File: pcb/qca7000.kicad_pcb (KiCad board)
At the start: 2 copper layers, 76 x 68.4 mm, 113 parts, among them J1 Conn_01x04_Pin, J2 Conn_01x08_Pin, J3 12V_in, U1 25Q16, U2 XL1509-5.0, U3 AMS1117-3.3, U4 AMS1117-3.3, Y1 25MHz

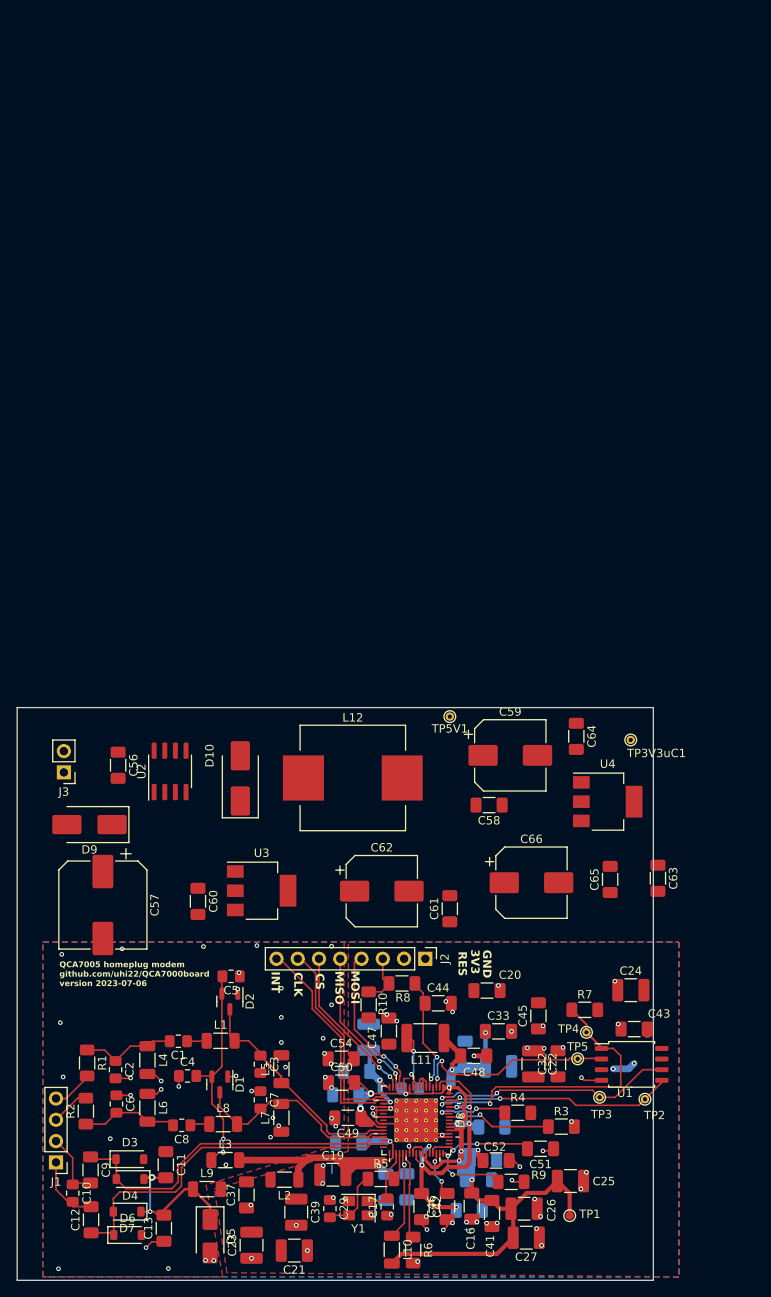
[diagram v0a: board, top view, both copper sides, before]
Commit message: added sheets for inputs and outputs. layout draft.
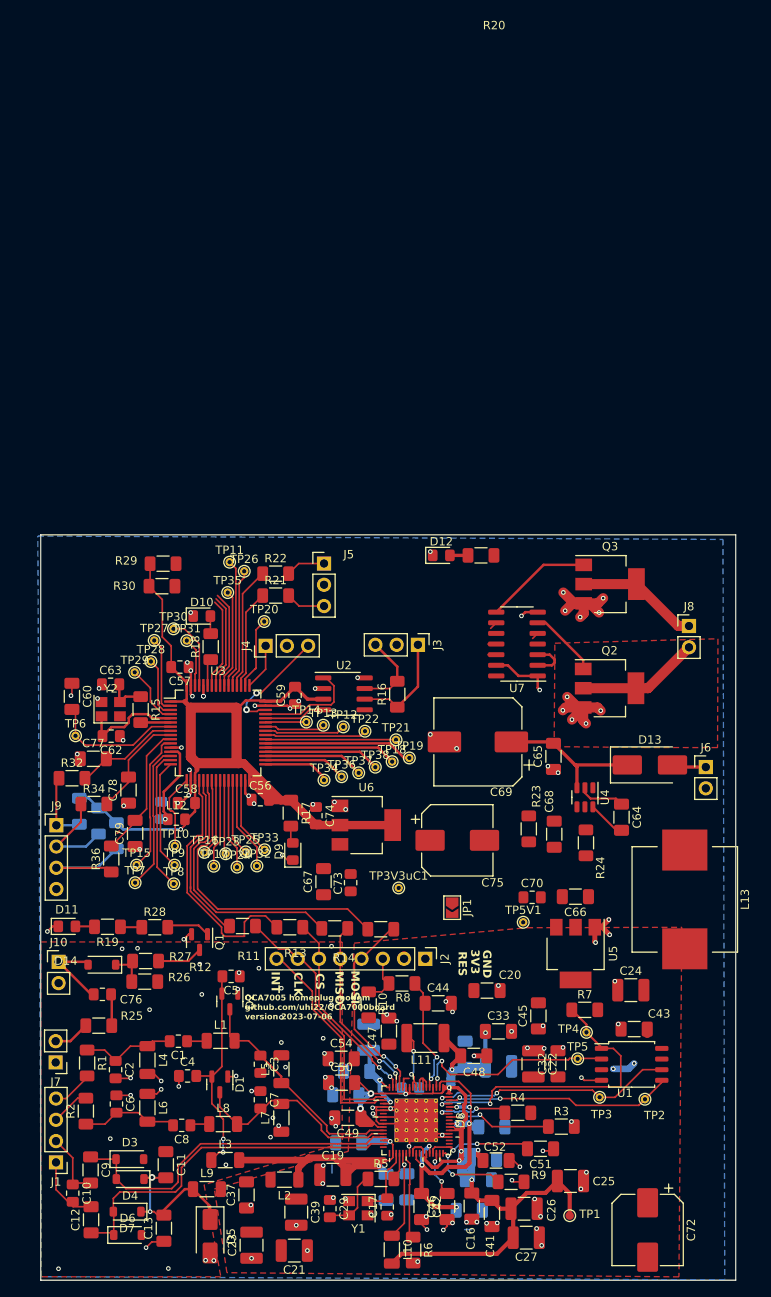
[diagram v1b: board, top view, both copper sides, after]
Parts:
- added C67: 22uF, Capacitor_SMD:C_1206_3216Metric_Pad1.33x1.80mm_HandSolder, F.Cu at (154.9, 81.5)
- added C68: 68pF, Capacitor_SMD:C_1206_3216Metric_Pad1.33x1.80mm_HandSolder, F.Cu at (182.5, 75.8)
- added C69: 470uF, Capacitor_SMD:CP_Elec_10x10, F.Cu at (173.4, 64.8)
- added C70: 100nF, Capacitor_SMD:C_0805_2012Metric_Pad1.18x1.45mm_HandSolder, F.Cu at (179.8, 83.3)
- added C72: 100uF, Capacitor_SMD:CP_Elec_8x10, F.Cu at (193.6, 123.1)
- added C73: 100nF, Capacitor_SMD:C_0805_2012Metric_Pad1.18x1.45mm_HandSolder, F.Cu at (158.2, 81.6)
- added C74: 100nF, Capacitor_SMD:C_0805_2012Metric_Pad1.18x1.45mm_HandSolder, F.Cu at (154.0, 73.6)
- added C75: 100uF, Capacitor_SMD:CP_Elec_8x10, F.Cu at (170.9, 76.5)
- added C76: 1nF, Capacitor_SMD:C_0805_2012Metric_Pad1.18x1.45mm_HandSolder, F.Cu at (128.5, 94.9)
- added C77: 100nF, Capacitor_SMD:C_1206_3216Metric_Pad1.33x1.80mm_HandSolder, F.Cu at (127.4, 66.8)
- added C78: 100nF, Capacitor_SMD:C_1206_3216Metric_Pad1.33x1.80mm_HandSolder, F.Cu at (131.6, 70.5)
- added C79: 100nF, Capacitor_SMD:C_1206_3216Metric_Pad1.33x1.80mm_HandSolder, F.Cu at (132.4, 75.7)
- added D11: LED, LED_SMD:LED_0805_2012Metric_Pad1.15x1.40mm_HandSolder, F.Cu at (124.3, 86.8)
- added D12: LED, LED_SMD:LED_0805_2012Metric_Pad1.15x1.40mm_HandSolder, F.Cu at (169.0, 42.5)
- added D13: SS54B-HF, Diode_SMD:D_SMB_Handsoldering, F.Cu at (193.9, 67.5)
- added D14: 1N4148W, Diode_SMD:D_SOD-123, F.Cu at (128.4, 91.4)
- added J10: CP/PE, Connector_PinHeader_2.54mm:PinHeader_1x02_P2.54mm_Vertical, F.Cu at (123.3, 91.0)
- added J4: DEBUG, Connector_PinHeader_2.54mm:PinHeader_1x03_P2.54mm_Vertical, F.Cu at (148.0, 53.3)
- added J5: UART, Connector_PinHeader_2.54mm:PinHeader_1x03_P2.54mm_Vertical, F.Cu at (155.0, 43.5)
- added J6: 12V_in, Connector_PinHeader_2.54mm:PinHeader_1x02_P2.54mm_Vertical, F.Cu at (200.6, 67.8)
- added J7: RF, Connector_PinHeader_2.54mm:PinHeader_1x02_P2.54mm_Vertical, F.Cu at (122.9, 103.1)
- added J8: CONTACTORS, Connector_PinHeader_2.54mm:PinHeader_1x02_P2.54mm_Vertical, F.Cu at (198.6, 50.9)
- added J9: Temps, Connector_PinHeader_2.54mm:PinHeader_1x04_P2.54mm_Vertical, F.Cu at (123.0, 74.7)
- added JP1: SolderJumper3V3together, Jumper:SolderJumper-2_P1.3mm_Open_TrianglePad1.0x1.5mm, F.Cu at (170.3, 84.6)
- added L13: 10uH, Inductor_SMD:L_Wuerth_WE-PD-Typ-LS_Handsoldering, F.Cu at (198.1, 83.6)
- added Q1: BC846, Package_TO_SOT_SMD:SOT-23, F.Cu at (140.1, 88.7)
- added Q2: NCV8402xST, Package_TO_SOT_SMD:SOT-223, F.Cu at (189.1, 58.4)
- added Q3: NCV8402xST, Package_TO_SOT_SMD:SOT-223, F.Cu at (189.2, 45.9)
- added R11: 220, Resistor_SMD:R_1206_3216Metric_Pad1.30x1.75mm_HandSolder, F.Cu at (150.9, 86.9)
- added R12: 220, Resistor_SMD:R_1206_3216Metric_Pad1.30x1.75mm_HandSolder, F.Cu at (145.2, 86.8)
- added R13: 220, Resistor_SMD:R_1206_3216Metric_Pad1.30x1.75mm_HandSolder, F.Cu at (156.3, 87.0)
- added R14: 220, Resistor_SMD:R_1206_3216Metric_Pad1.30x1.75mm_HandSolder, F.Cu at (161.8, 87.2)
- added R15: 33, Resistor_SMD:R_1206_3216Metric_Pad1.30x1.75mm_HandSolder, F.Cu at (133.1, 60.9)
- added R16: 1k, Resistor_SMD:R_1206_3216Metric_Pad1.30x1.75mm_HandSolder, F.Cu at (163.7, 59.1)
- added R17: 1k, Resistor_SMD:R_1206_3216Metric_Pad1.30x1.75mm_HandSolder, F.Cu at (151.0, 73.3)
- added R18: 1k, Resistor_SMD:R_1206_3216Metric_Pad1.30x1.75mm_HandSolder, F.Cu at (141.4, 53.4)
- added R19: 1k, Resistor_SMD:R_1206_3216Metric_Pad1.30x1.75mm_HandSolder, F.Cu at (129.1, 86.9)
- added R20: 1k, Resistor_SMD:R_1206_3216Metric_Pad1.30x1.75mm_HandSolder, F.Cu at (173.7, 42.5)
- added R21: 220, Resistor_SMD:R_1206_3216Metric_Pad1.30x1.75mm_HandSolder, F.Cu at (149.2, 47.3)
- added R22: 220, Resistor_SMD:R_1206_3216Metric_Pad1.30x1.75mm_HandSolder, F.Cu at (149.2, 44.7)
- added R23: 10k, Resistor_SMD:R_1206_3216Metric_Pad1.30x1.75mm_HandSolder, F.Cu at (179.4, 75.2)
- added R24: 10k, Resistor_SMD:R_1206_3216Metric_Pad1.30x1.75mm_HandSolder, F.Cu at (186.3, 76.8)
- added R25: 180, Resistor_SMD:R_1206_3216Metric_Pad1.30x1.75mm_HandSolder, F.Cu at (128.1, 98.7)
- added R26: 2k7, Resistor_SMD:R_1206_3216Metric_Pad1.30x1.75mm_HandSolder, F.Cu at (133.6, 93.4)
- added R27: 1k2, Resistor_SMD:R_1206_3216Metric_Pad1.30x1.75mm_HandSolder, F.Cu at (133.7, 91.0)
- added R28: 10k, Resistor_SMD:R_1206_3216Metric_Pad1.30x1.75mm_HandSolder, F.Cu at (134.8, 86.9)
- added R29: 10k, Resistor_SMD:R_1206_3216Metric_Pad1.30x1.75mm_HandSolder, F.Cu at (135.8, 43.5)
- added R30: 10k, Resistor_SMD:R_1206_3216Metric_Pad1.30x1.75mm_HandSolder, F.Cu at (135.6, 46.2)
- added R31: 10k, Resistor_SMD:R_1206_3216Metric_Pad1.30x1.75mm_HandSolder, B.Cu at (125.8, 73.0)
- added R32: 47k, Resistor_SMD:R_1206_3216Metric_Pad1.30x1.75mm_HandSolder, F.Cu at (124.9, 69.1)
- added R33: 10k, Resistor_SMD:R_1206_3216Metric_Pad1.30x1.75mm_HandSolder, B.Cu at (128.0, 74.2)
- added R34: 47k, Resistor_SMD:R_1206_3216Metric_Pad1.30x1.75mm_HandSolder, F.Cu at (127.5, 72.2)
- added R35: 10k, Resistor_SMD:R_1206_3216Metric_Pad1.30x1.75mm_HandSolder, B.Cu at (130.2, 76.0)
- added R36: 47k, Resistor_SMD:R_1206_3216Metric_Pad1.30x1.75mm_HandSolder, F.Cu at (129.6, 78.8)
- added TP10: ~, TestPoint:TestPoint_THTPad_D1.0mm_Drill0.5mm, F.Cu at (137.2, 77.2)
- added TP11: ~, TestPoint:TestPoint_THTPad_D1.0mm_Drill0.5mm, F.Cu at (143.7, 43.3)
- added TP12: ~, TestPoint:TestPoint_THTPad_D1.0mm_Drill0.5mm, F.Cu at (157.3, 63.0)
- added TP13: ~, TestPoint:TestPoint_THTPad_D1.0mm_Drill0.5mm, F.Cu at (154.9, 62.8)
- added TP14: ~, TestPoint:TestPoint_THTPad_D1.0mm_Drill0.5mm, F.Cu at (152.9, 62.4)
- added TP15: ~, TestPoint:TestPoint_THTPad_D1.0mm_Drill0.5mm, F.Cu at (132.6, 79.5)
- added TP16: ~, TestPoint:TestPoint_THTPad_D1.0mm_Drill0.5mm, F.Cu at (140.7, 78.0)
- added TP17: ~, TestPoint:TestPoint_THTPad_D1.0mm_Drill0.5mm, F.Cu at (141.8, 79.6)
- added TP18: ~, TestPoint:TestPoint_THTPad_D1.0mm_Drill0.5mm, F.Cu at (163.1, 67.1)
- added TP19: ~, TestPoint:TestPoint_THTPad_D1.0mm_Drill0.5mm, F.Cu at (165.2, 66.7)
- added TP20: ~, TestPoint:TestPoint_THTPad_D1.0mm_Drill0.5mm, F.Cu at (147.8, 50.4)
- added TP21: ~, TestPoint:TestPoint_THTPad_D1.0mm_Drill0.5mm, F.Cu at (163.6, 64.5)
- added TP22: ~, TestPoint:TestPoint_THTPad_D1.0mm_Drill0.5mm, F.Cu at (159.9, 63.5)
- added TP23: ~, TestPoint:TestPoint_THTPad_D1.0mm_Drill0.5mm, F.Cu at (143.2, 78.1)
- added TP24: ~, TestPoint:TestPoint_THTPad_D1.0mm_Drill0.5mm, F.Cu at (144.6, 79.7)
- added TP25: ~, TestPoint:TestPoint_THTPad_D1.0mm_Drill0.5mm, F.Cu at (145.6, 77.9)
- added TP26: ~, TestPoint:TestPoint_THTPad_D1.0mm_Drill0.5mm, F.Cu at (145.4, 44.4)
- added TP27: ~, TestPoint:TestPoint_THTPad_D1.0mm_Drill0.5mm, F.Cu at (134.7, 52.6)
- added TP28: ~, TestPoint:TestPoint_THTPad_D1.0mm_Drill0.5mm, F.Cu at (134.3, 55.2)
- added TP29: ~, TestPoint:TestPoint_THTPad_D1.0mm_Drill0.5mm, F.Cu at (132.4, 56.5)
- added TP30: ~, TestPoint:TestPoint_THTPad_D1.0mm_Drill0.5mm, F.Cu at (137.0, 51.3)
- added TP31: ~, TestPoint:TestPoint_THTPad_D1.0mm_Drill0.5mm, F.Cu at (138.6, 52.7)
- added TP32: ~, TestPoint:TestPoint_THTPad_D1.0mm_Drill0.5mm, F.Cu at (147.0, 79.6)
- added TP33: ~, TestPoint:TestPoint_THTPad_D1.0mm_Drill0.5mm, F.Cu at (147.9, 77.7)
- added TP34: ~, TestPoint:TestPoint_THTPad_D1.0mm_Drill0.5mm, F.Cu at (155.0, 69.3)
- added TP35: SWO, TestPoint:TestPoint_THTPad_D1.0mm_Drill0.5mm, F.Cu at (143.5, 46.9)
- added TP36: ~, TestPoint:TestPoint_THTPad_D1.0mm_Drill0.5mm, F.Cu at (157.1, 68.9)
- added TP37: ~, TestPoint:TestPoint_THTPad_D1.0mm_Drill0.5mm, F.Cu at (159.1, 68.5)
- added TP38: ~, TestPoint:TestPoint_THTPad_D1.0mm_Drill0.5mm, F.Cu at (161.1, 67.8)
- added TP6: uC_RESET, TestPoint:TestPoint_THTPad_D1.0mm_Drill0.5mm, F.Cu at (125.3, 64.0)
- added TP7: ~, TestPoint:TestPoint_THTPad_D1.0mm_Drill0.5mm, F.Cu at (132.4, 81.6)
- added TP8: ~, TestPoint:TestPoint_THTPad_D1.0mm_Drill0.5mm, F.Cu at (137.0, 81.7)
- added TP9: ~, TestPoint:TestPoint_THTPad_D1.0mm_Drill0.5mm, F.Cu at (137.1, 79.5)
- added U5: AMS1117-3.3, Package_TO_SOT_SMD:SOT-223-3_TabPin2, F.Cu at (185.0, 90.1)
- added U6: AMS1117-3.3, Package_TO_SOT_SMD:SOT-223-3_TabPin2, F.Cu at (160.0, 74.7)
- added U7: 74HCT04, Package_SO:SO-14_3.9x8.65mm_P1.27mm, F.Cu at (178.0, 53.1)
- added Y2: 8MHz, Crystal:Crystal_SMD_TXC_7M-4Pin_3.2x2.5mm, F.Cu at (129.5, 60.9)
- C56, C58: footprint Capacitor_SMD:C_1206_3216Metric_Pad1.33x1.80mm_HandSolder -> Capacitor_SMD:C_0805_2012Metric_Pad1.18x1.45mm_HandSolder
- C57: value 470uF -> 100nF; footprint Capacitor_SMD:CP_Elec_10x10 -> Capacitor_SMD:C_0805_2012Metric_Pad1.18x1.45mm_HandSolder
- C59: value 100uF -> 100nF; footprint Capacitor_SMD:CP_Elec_8x10 -> Capacitor_SMD:C_0805_2012Metric_Pad1.18x1.45mm_HandSolder
- C61: footprint Capacitor_SMD:C_1206_3216Metric_Pad1.33x1.80mm_HandSolder -> Capacitor_SMD:C_0805_2012Metric_Pad1.18x1.45mm_HandSolder; moved to B.Cu
- C62: value 100uF -> 22p; footprint Capacitor_SMD:CP_Elec_8x10 -> Capacitor_SMD:C_0805_2012Metric_Pad1.18x1.45mm_HandSolder
- C63: value 100nF -> 22p; footprint Capacitor_SMD:C_1206_3216Metric_Pad1.33x1.80mm_HandSolder -> Capacitor_SMD:C_0805_2012Metric_Pad1.18x1.45mm_HandSolder
- C65: value 100nF -> 10uF
- C66: value 100uF -> 22uF; footprint Capacitor_SMD:CP_Elec_8x10 -> Capacitor_SMD:C_1206_3216Metric_Pad1.33x1.80mm_HandSolder
- D10, D9: value SS54B-HF -> LED; footprint Diode_SMD:D_SMB_Handsoldering -> LED_SMD:LED_0805_2012Metric_Pad1.15x1.40mm_HandSolder
- J3: value 12V_in -> CAN; footprint Connector_PinHeader_2.54mm:PinHeader_1x02_P2.54mm_Vertical -> Connector_PinHeader_2.54mm:PinHeader_1x03_P2.54mm_Vertical
- L12: value 68uH -> Bead 600; footprint Inductor_SMD:L_Wuerth_WE-PD-Typ-LS_Handsoldering -> Inductor_SMD:L_0805_2012Metric_Pad1.15x1.40mm_HandSolder
- R6: value 2.5k -> 6k2
- U2: value XL1509-5.0 -> SN65HVD234
- U3: value AMS1117-3.3 -> STM32F103RETx; footprint Package_TO_SOT_SMD:SOT-223-3_TabPin2 -> Package_QFP:LQFP-64_10x10mm_P0.5mm
- U4: value AMS1117-3.3 -> TPS54302; footprint Package_TO_SOT_SMD:SOT-223-3_TabPin2 -> Package_TO_SOT_SMD:SOT-23-6
- moved C63 69.4 mm to (129.5, 57.9), turned to 0 degrees
- moved J3 45.0 mm to (166.2, 53.2), turned to -90 degrees
- moved C62 37.3 mm to (129.6, 64.1), turned to 180 degrees
- moved C61 36.4 mm to (135.5, 73.0), turned to -90 degrees
- moved C58 36.2 mm to (138.5, 72.1), turned to 0 degrees
- moved TP3V3uC1 32.9 mm to (163.9, 82.2), turned to 0 degrees
- moved C57 29.9 mm to (137.8, 55.8), turned to 180 degrees
- moved C60 28.8 mm to (124.9, 59.3)
- moved C59 26.7 mm to (151.5, 59.2), turned to 90 degrees
- moved TP5V1 26.1 mm to (178.8, 86.3), turned to 0 degrees
- moved D9 24.5 mm to (151.2, 77.9), turned to 90 degrees
- moved U2 22.7 mm to (157.4, 59.0), turned to 0 degrees
- moved L12 21.7 mm to (137.3, 74.0)
- moved D10 19.9 mm to (140.4, 49.7), turned to 0 degrees
- moved U3 19.6 mm to (142.3, 63.7)
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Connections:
- C56 pad 2: 12V_P -> 3V3_uC
- C57 pad 1: 12V_P -> GND
- C57 pad 2: GND -> 3V3_uC
- C58 pad 2: 5V -> 3V3_uC
- C59 pad 1: 5V -> GND
- C59 pad 2: GND -> 3V3_uC
- C60 pad 2: 5V -> uC_RESET
- C61 pad 2: 3V3_D -> Net-(U3-VDDA)
- C62 pad 1: 3V3_D -> GND
- C62 pad 2: GND -> /controller/OCS_IN
- C63 pad 1: 3V3_uC -> GND
- C63 pad 2: GND -> Net-(C63-Pad2)
- C64 pad 1: GND -> Net-(U4-SW)
- C64 pad 2: 5V -> Net-(U4-BOOT)
- C65 pad 2: 3V3_uC -> 12V_P
- C66 pad 1: 3V3_uC -> GND
- C66 pad 2: GND -> 5V
- D10 pad 1: Net-(D10-K) -> GND
- D10 pad 2: GND -> Net-(D10-A)
- D9 pad 1: 12V_P -> GND
- D9 pad 2: 12V -> Net-(D9-A)
- J3 pad 1: 12V -> CANL
- L12 pad 1: Net-(D10-K) -> Net-(U3-VDDA)
- L12 pad 2: 5V -> 3V3_uC
- R10 pad 2: +3V3_D -> 3V3_D
- R4 pad 2: +3V3_D -> 3V3_D
- U2 pad 1: 12V_P -> CAN_TX
- U2 pad 2: Net-(D10-K) -> GND
- U2 pad 3: 5V -> 3V3_uC
- U2 pad 4: GND -> CAN_RX
- U2 pad 5: GND -> unconnected-(U2-EN-Pad5)
- U2 pad 6: GND -> CANL
- U2 pad 7: GND -> CANH
- U3 pad 1: GND -> 3V3_uC
- U3 pad 2: 3V3_D -> Net-(U3-PC13)
- U3 pad 3: 5V -> Net-(U3-PC14)
- U4 pad 2: 3V3_uC -> Net-(U4-SW)
- U4 pad 3: 5V -> 12V_P
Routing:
- net 3V3_uC: track 0.00 -> 125.3 mm, vias 0 -> 1
- net GND: track 63.9 -> 127.7 mm, vias 86 -> 136
- net SPI1_MOSI: track 0.00 -> 36.4 mm
- net SPI1_MISO: track 0.00 -> 31.4 mm
- net SPI1_NSS: track 0.00 -> 30.5 mm
- net SPI1_CLK: track 0.00 -> 21.0 mm
- net Net-(U3-PC7): track 0.00 -> 17.9 mm
- net 12V_P: track 0.00 -> 17.8 mm
- net Net-(U3-PA0): track 0.00 -> 17.5 mm
- net Net-(U3-PA1): track 0.00 -> 16.8 mm
- net Net-(U3-PC3): track 0.00 -> 16.7 mm
- net ADC123_IN12: track 0.00 -> 16.2 mm
- net uC_RESET: track 0.00 -> 16.1 mm
- net Net-(U3-PC6): track 0.00 -> 15.8 mm
- net Net-(U3-PC8): track 0.00 -> 15.7 mm
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- added copper zone on F.Cu, net 3V3_D
- added copper zone on F.Cu, net CONTACTOR1_LS
- removed copper zone on F.Cu, net +3V3_D
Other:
- board size 76 x 68.4 mm -> 83 x 89 mm

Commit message: layout for stm, supply, drivers, flash programming connector
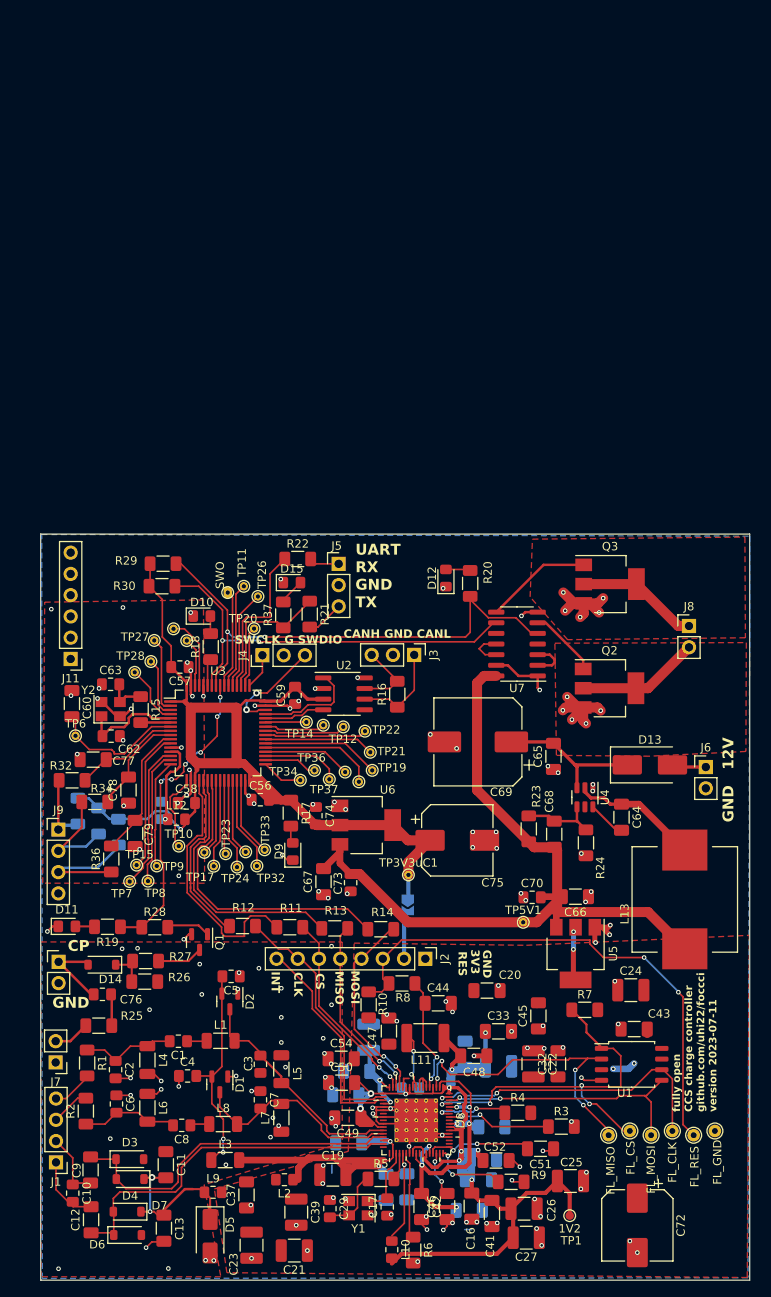
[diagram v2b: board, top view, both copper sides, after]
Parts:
- added D15: UARTTX, LED_SMD:LED_0805_2012Metric_Pad1.15x1.40mm_HandSolder, F.Cu at (151.1, 45.7)
- added J11: spare, Connector_PinHeader_2.54mm:PinHeader_1x06_P2.54mm_Vertical, F.Cu at (124.7, 54.9)
- added R37: 1k, Resistor_SMD:R_1206_3216Metric_Pad1.30x1.75mm_HandSolder, F.Cu at (150.1, 49.6)
- added TP39: FL_GND, TestPoint:TestPoint_THTPad_D1.5mm_Drill0.7mm, F.Cu at (201.7, 111.3)
- added TP40: FL_RES, TestPoint:TestPoint_THTPad_D1.5mm_Drill0.7mm, F.Cu at (199.1, 111.8)
- D10: value LED -> ALIVE
- D11: value LED -> STATEC
- D12: value LED -> CONTACTOR1
- D9: value LED -> PWR
- JP1: moved to B.Cu
- L10, L2, L9: footprint Inductor_SMD:L_1206_3216Metric_Pad1.22x1.90mm_HandSolder -> Inductor_SMD:L_0805_2012Metric_Pad1.15x1.40mm_HandSolder
- TP2, TP3, TP4, TP5: footprint TestPoint:TestPoint_THTPad_D1.0mm_Drill0.5mm -> TestPoint:TestPoint_THTPad_D1.5mm_Drill0.7mm
- moved TP4 12.9 mm to (191.5, 111.3)
- moved TP5 9.85 mm to (189.0, 111.8)
- moved TP3 9.58 mm to (196.6, 111.3)
- moved JP1 5.32 mm to (165.0, 84.2)
- moved TP19 4.67 mm to (160.7, 68.2)
- moved TP18 4.65 mm to (159.1, 69.5)
- moved R21 4.63 mm to (153.3, 49.5), turned to -90 degrees
- moved TP2 4.36 mm to (194.1, 111.8)
- moved TP38 3.66 mm to (157.5, 68.4)
- moved TP37 3.59 mm to (155.6, 69.2)
- moved R20 3.59 mm to (172.4, 45.8), turned to 90 degrees
- moved TP26 3.42 mm to (147.1, 47.4)
- moved TP21 3.41 mm to (160.5, 66.0)
- moved TP11 3.34 mm to (145.4, 46.2)
- moved TP36 3.33 mm to (153.8, 68.2)
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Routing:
- net 5V: track 0.00 -> 94.8 mm
- net RESET#: track 6.30 -> 63.3 mm, vias 0 -> 2
- net CONTACTOR_CONTROL1: track 12.2 -> 61.9 mm, vias 0 -> 2
- net CONTACTOR_CONTROL2: track 11.8 -> 50.1 mm, vias 0 -> 2
- net STATE_C_CONTROL: track 14.3 -> 36.8 mm, vias 0 -> 6
- net 3V3_uC: track 125.3 -> 139.0 mm
- net 3V3_D: track 58.5 -> 70.8 mm, vias 11 -> 13
- net SPI_DI: track 24.5 -> 36.0 mm, vias 2 -> 4
- net Net-(U4-SW): track 5.54 -> 15.9 mm
- net Net-(U4-FB): track 0.00 -> 9.23 mm
- net SPI_CS_L: track 36.5 -> 45.4 mm, vias 2 -> 4
- net SPI_CLK: track 29.5 -> 36.8 mm
- net UART4_TX: track 11.8 -> 17.0 mm
- net UART4_RX: track 14.6 -> 19.1 mm
- net SPI_DO: track 27.3 -> 31.6 mm
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- added copper zone on F.Cu, net CONTACTOR2_LS
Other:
- board size 83 x 89 mm -> 84.7 x 89.1 mm
- board text added: "CANH GND CANL"
- board text added: "CP"
- board text added: "GND 12V"
- board text added: "SWCLK G SWDIO"
- board text added: "UART RX GND TX"
- board text added: "fully open CCS charge controller github.com/uhi22/foccci version 2023-07-11"
- board text removed: "QCA7005 homeplug modem github.com/uhi22/QCA7000board version 2023-07-06"
